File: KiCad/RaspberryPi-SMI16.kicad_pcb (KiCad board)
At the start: 2 copper layers, 86 x 133.5 mm, 20 parts, among them J1 Screw_Terminal_01x02, U1 RASPBERRYPI_GPIO_40, U2 RFID-RC522

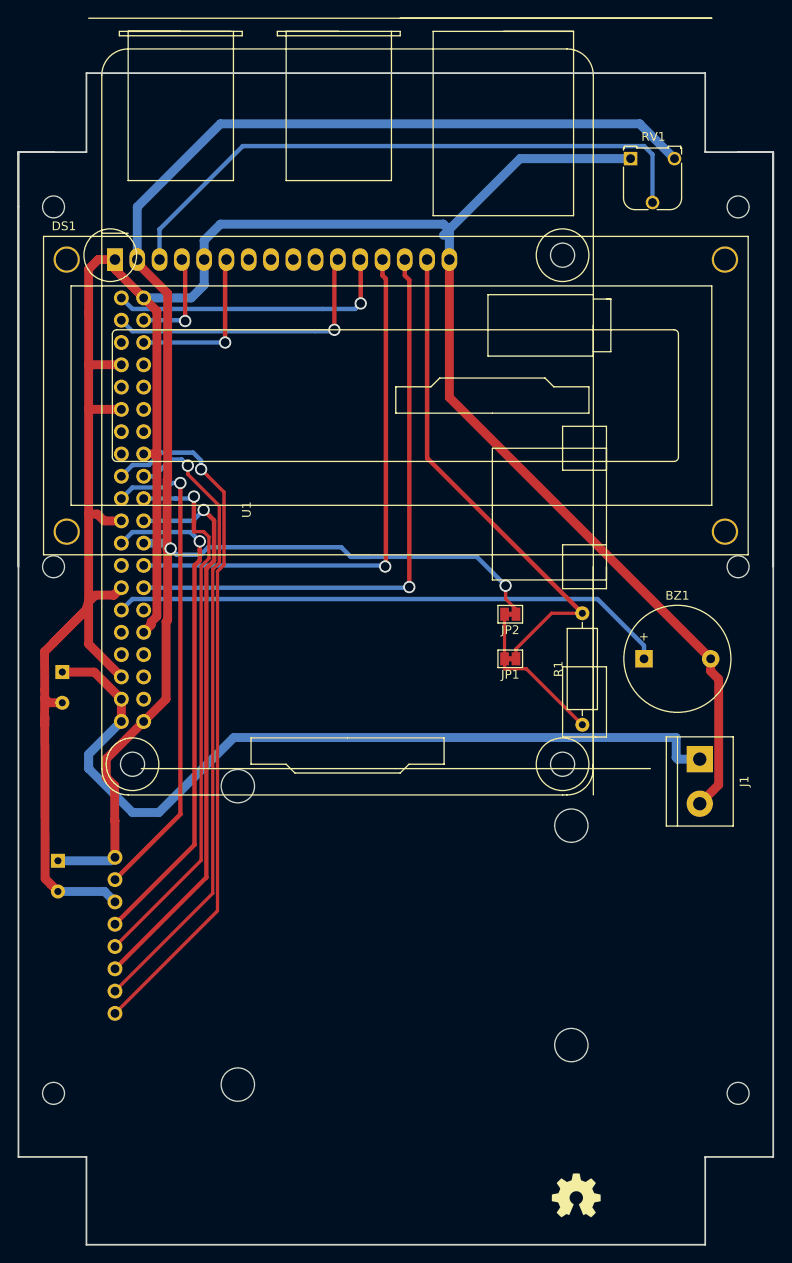
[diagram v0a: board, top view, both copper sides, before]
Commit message: change KiCad7
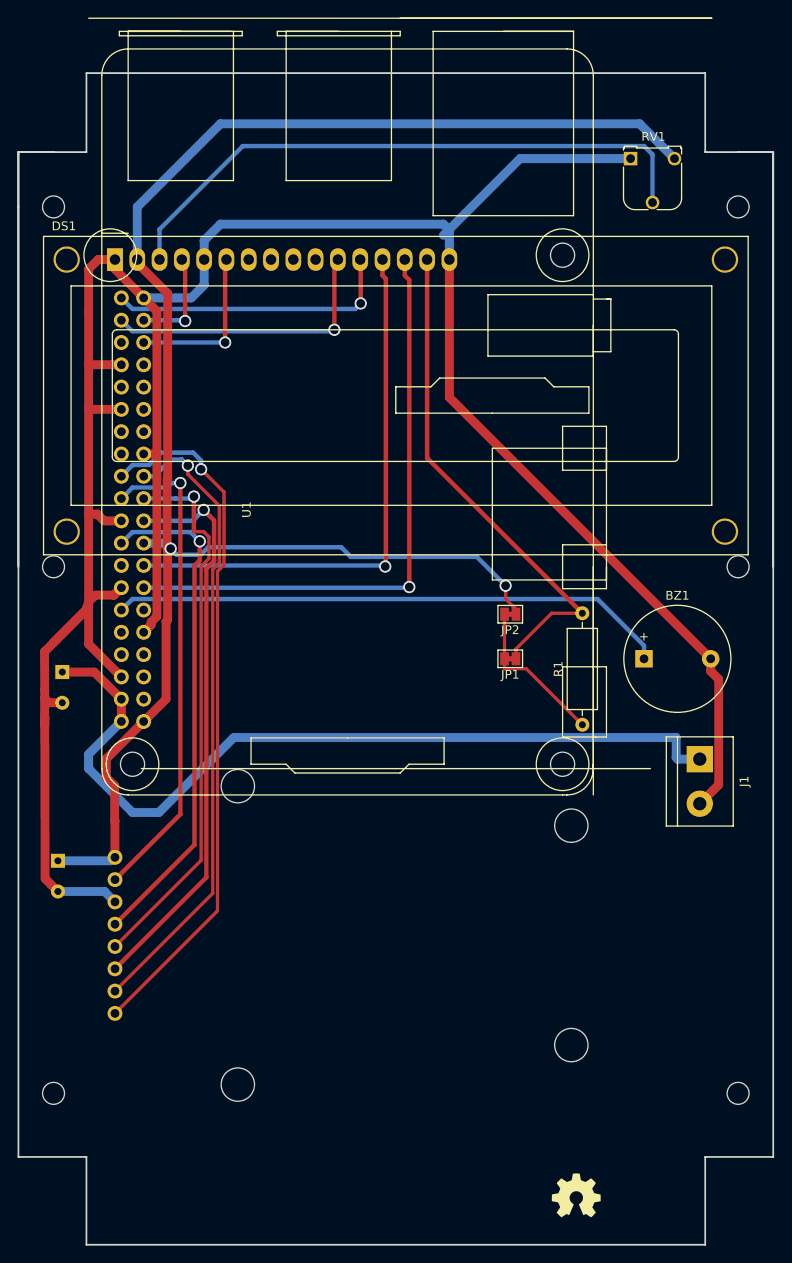
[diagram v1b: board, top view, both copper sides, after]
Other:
- net class Default removed
